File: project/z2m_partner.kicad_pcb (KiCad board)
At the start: 2 copper layers, 50 x 50 mm, 34 parts, among them J1 Conn_01x05, SW1 SW_DIP_x02, SW2 SW_Push, SW3 SW_Push, U1 CH340G, U2 CD4052B, U3 E18-MS1-PCB, U4 74LVC1G66, U5 74LVC1G66, U6 AP1117-33, U7 ESP-WROOM-02, Y1 12MHz

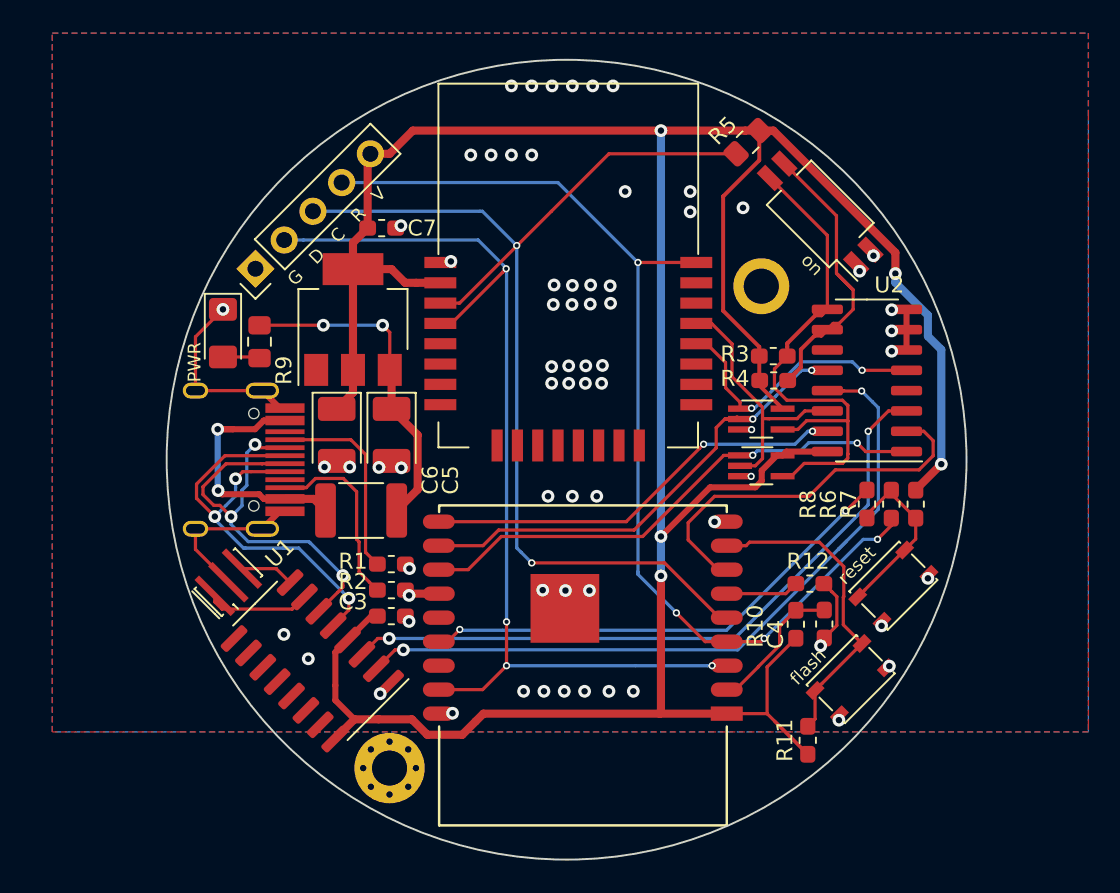
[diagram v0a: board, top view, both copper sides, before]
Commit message: Update to v02
Signed-off-by: SchumyHao <schumyhaojl@126.com>
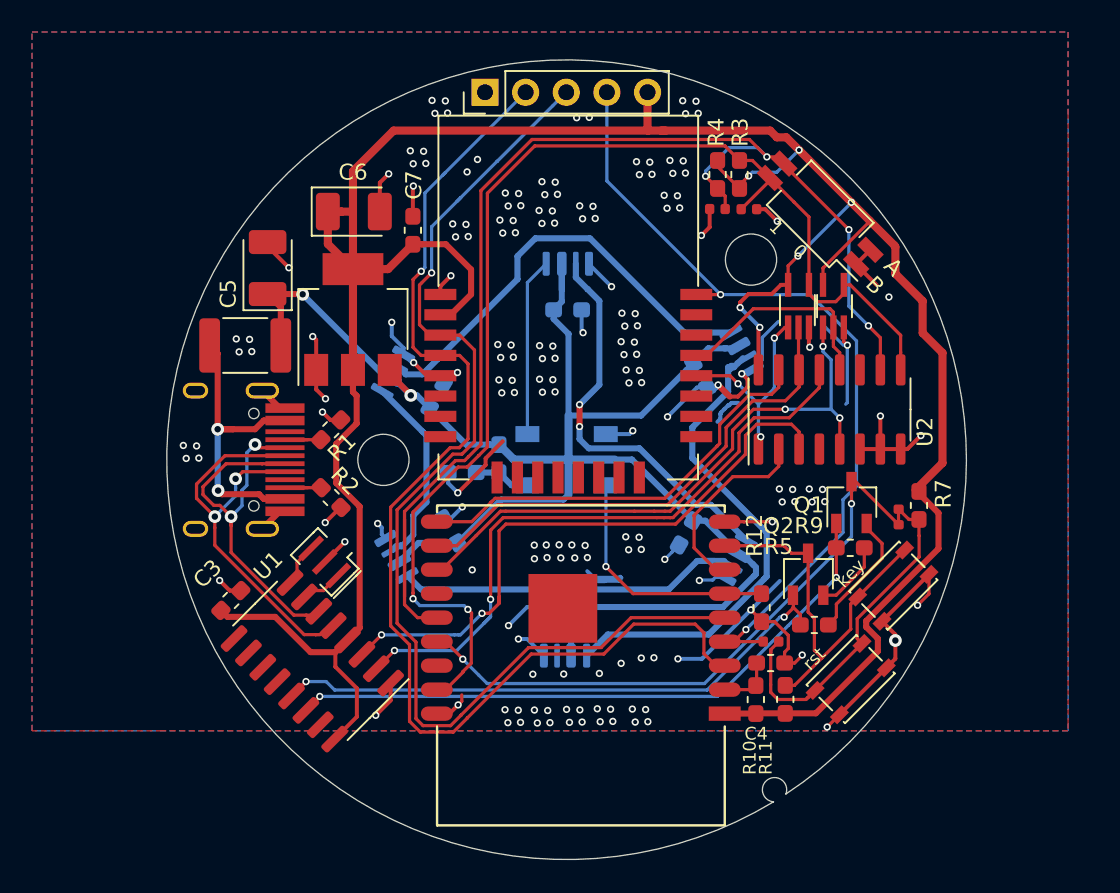
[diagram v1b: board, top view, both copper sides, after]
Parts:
- removed the REF** at (173.5, 122.1)
- removed the REF** at (196.7, 92.0)
- added C1: 100nF, Capacitor_SMD:C_0603_1608Metric_Pad1.05x0.95mm_HandSolder, B.Cu at (178.0, 103.7)
- added C10: 100nF, Capacitor_SMD:C_0603_1608Metric_Pad1.05x0.95mm_HandSolder, B.Cu at (192.9, 97.6)
- added C11: 100nF, Capacitor_SMD:C_0603_1608Metric_Pad1.05x0.95mm_HandSolder, B.Cu at (184.5, 112.1)
- added C12: 100nF, Capacitor_SMD:C_0603_1608Metric_Pad1.05x0.95mm_HandSolder, B.Cu at (176.4, 98.9)
- added C2: 100nF, Capacitor_SMD:C_0603_1608Metric_Pad1.05x0.95mm_HandSolder, B.Cu at (184.6, 93.5)
- added C8: 100nF, Capacitor_SMD:C_0603_1608Metric_Pad1.05x0.95mm_HandSolder, B.Cu at (177.3, 107.3)
- added C9: 100nF, Capacitor_SMD:C_0603_1608Metric_Pad1.05x0.95mm_HandSolder, B.Cu at (192.0, 107.4)
- added D2: D, Diode_SMD:D_0603_1608Metric_Pad1.05x0.95mm_HandSolder, B.Cu at (180.3, 102.8)
- added D3: WS2812B, z2m_partner:SK6812_4020, B.Cu at (184.6, 89.9)
- added D4: WS2812B, z2m_partner:SK6812_4020, B.Cu at (173.3, 109.4)
- added D5: WS2812B, z2m_partner:SK6812_4020, B.Cu at (195.8, 109.4)
- added D6: WS2812B, z2m_partner:SK6812_4020, B.Cu at (173.0, 97.1)
- added D7: WS2812B, z2m_partner:SK6812_4020, B.Cu at (196.1, 95.7)
- added D8: WS2812B, z2m_partner:SK6812_4020, B.Cu at (184.5, 115.9)
- added Q1: S8050, Package_TO_SOT_SMD:TSOT-23, F.Cu at (202.4, 105.5)
- added Q2: S8050, Package_TO_SOT_SMD:TSOT-23, F.Cu at (199.7, 110.0)
- added R13: 0-NC, Resistor_SMD:R_0402_1005Metric, F.Cu at (195.9, 87.2)
- added R14: 0-NC, Resistor_SMD:R_0402_1005Metric, F.Cu at (194.0, 87.2)
- added REF**: MountingHole_3.2mm_M3_ISO14580, MountingHole:MountingHole_3.2mm_M3_ISO14580, F.Cu at (196.1, 90.4)
- added REF**: MountingHole_3.2mm_M3_ISO14580, MountingHole:MountingHole_3.2mm_M3_ISO14580, F.Cu at (173.1, 102.9)
- D1: value LED -> WS2812B; footprint LED_SMD:LED_1206_3216Metric_Pad1.42x1.75mm_HandSolder -> LED_SMD:LED_WS2812B_PLCC4_5.0x5.0mm_P3.2mm; moved to B.Cu
- R3, R4: value 10k -> 10k-NC
- R5, R9: value 1k -> 12k; footprint Resistor_SMD:R_0805_2012Metric_Pad1.15x1.40mm_HandSolder -> Resistor_SMD:R_0603_1608Metric_Pad1.05x0.95mm_HandSolder
- R6, R8: footprint Resistor_SMD:R_0603_1608Metric_Pad1.05x0.95mm_HandSolder -> Resistor_SMD:R_0402_1005Metric
- Y1: footprint Crystal:Resonator_SMD_muRata_CSTxExxV-3Pin_3.0x1.1mm_HandSoldering -> Crystal:Resonator_SMD_muRata_CSTxExxV-3Pin_3.0x1.1mm
- moved R9 39.1 mm to (202.3, 108.4), turned to 0 degrees
- moved R5 30.5 mm to (200.0, 113.2), turned to 0 degrees
- moved D1 22.9 mm to (184.6, 102.9), turned to 0 degrees
- moved J1 18.1 mm to (179.4, 79.9), turned to 90 degrees
- moved C6 14.0 mm to (171.2, 87.4), turned to 0 degrees
- moved R4 13.3 mm to (194.0, 85.0), turned to 270 degrees
- moved C5 13.0 mm to (165.9, 90.9), turned to 90 degrees
- moved F1 12.6 mm to (164.5, 95.7)
- moved R3 11.5 mm to (195.4, 85.0), turned to 90 degrees
- moved R6 11.4 mm to (197.3, 114.2), turned to 180 degrees
- moved U5 11.0 mm to (201.2, 93.3), turned to 90 degrees
- moved C3 10.1 mm to (163.6, 111.7), turned to 45 degrees
- moved R1 9.21 mm to (169.8, 101.0), turned to 225 degrees
- moved U4 7.43 mm to (199.1, 93.3), turned to 90 degrees
- moved R2 6.91 mm to (169.8, 105.2), turned to 135 degrees
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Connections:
- net Net-(R11-Pad2) renamed /ESP_IO0
- D1 pad 1: GND -> Net-(C1-Pad2)
- R12 pad 1: Net-(R12-Pad1) -> /LED
- R5 pad 1: +3V3 -> /DTR
- R5 pad 2: /E18_P22 -> Net-(Q1-Pad2)
- R9 pad 1: Net-(D1-Pad2) -> /RTS
- R9 pad 2: +5V -> Net-(Q2-Pad2)
- U1 pad 10: (no net) -> Net-(U1-Pad10)
- U1 pad 11: (no net) -> Net-(U1-Pad11)
- U1 pad 12: (no net) -> Net-(U1-Pad12)
- U1 pad 13: (no net) -> /DTR
- U1 pad 14: (no net) -> /RTS
- U1 pad 15: (no net) -> Net-(U1-Pad15)
- U1 pad 9: (no net) -> Net-(U1-Pad9)
- U2 pad 1: /ESP_TX -> /E18_TX
- U2 pad 11: (no net) -> Net-(U2-Pad11)
- U2 pad 12: /ESP_RX -> /E18_RX
- U2 pad 14: /E18_RX -> /ESP_RX
- U2 pad 4: (no net) -> Net-(U2-Pad4)
- U2 pad 5: /E18_TX -> /ESP_TX
- U3 pad 10: (no net) -> Net-(U3-Pad10)
- U3 pad 11: (no net) -> Net-(U3-Pad11)
- U3 pad 12: (no net) -> Net-(U3-Pad12)
- U3 pad 13: (no net) -> Net-(U3-Pad13)
- U3 pad 14: (no net) -> Net-(U3-Pad14)
- U3 pad 15: (no net) -> Net-(U3-Pad15)
- U3 pad 16: (no net) -> Net-(U3-Pad16)
- U3 pad 17: (no net) -> Net-(U3-Pad17)
- U3 pad 18: (no net) -> Net-(U3-Pad18)
- U3 pad 19: (no net) -> Net-(U3-Pad19)
- U3 pad 22: (no net) -> Net-(U3-Pad22)
- U3 pad 23: (no net) -> Net-(U3-Pad23)
- U3 pad 6: (no net) -> Net-(U3-Pad6)
- U3 pad 7: (no net) -> Net-(U3-Pad7)
- U3 pad 8: (no net) -> Net-(U3-Pad8)
- U3 pad 9: (no net) -> Net-(U3-Pad9)
- U7 pad 14: (no net) -> /SEL0
- U7 pad 16: (no net) -> Net-(U7-Pad16)
- U7 pad 17: /E18_P21 -> /SEL1
- U7 pad 6: Net-(R12-Pad1) -> /LED
- U7 pad PAD: GND -> (no net)
- USB1 pad 3: (no net) -> Net-(USB1-Pad3)
- USB1 pad 9: (no net) -> Net-(USB1-Pad9)
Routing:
- net GND: track 30.9 -> 122.1 mm, vias 69 -> 179
- net +5V: track 20.7 -> 100.1 mm
- net /SEL0: track 18.8 -> 79.3 mm, vias 0 -> 4
- net /SEL1: track 33.4 -> 79.8 mm, vias 0 -> 2
- net /RTS: track 0.00 -> 40.0 mm, vias 0 -> 2
- net /DTR: track 0.00 -> 36.2 mm, vias 0 -> 2
- net Net-(D7-Pad2): track 0.00 -> 30.6 mm
- net Net-(D6-Pad2): track 0.00 -> 27.9 mm
- net Net-(D3-Pad2): track 0.00 -> 25.1 mm, vias 0 -> 2
- net Net-(D4-Pad4): track 0.00 -> 21.7 mm
- net +3V3: track 195.6 -> 177.7 mm, vias 5 -> 6
- net /LED: track 0.00 -> 15.5 mm, vias 0 -> 1
- net /E18_RST: track 66.0 -> 53.4 mm, vias 4 -> 2
- net Net-(D4-Pad2): track 0.00 -> 12.2 mm
- net Net-(R6-Pad1): track 11.2 -> 22.6 mm
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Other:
- outline, holes or cut-outs redrawn
- rule via_min_drill: 0.3 -> 0.24
- rule via_min_size: 0.1778 -> 0.2
- board text added: "A B"
- board text added: "z2m partner v02"
- board text removed: "TTY control 00 USB<=>ESP ZB<=>NC 01 USB<=>ZB ESP<=>NC 10 ESP<=>ZB USB<=>DBG 11 ESP<=>ZB USB<=>NC"
- board text removed: "z2m partner v01"
